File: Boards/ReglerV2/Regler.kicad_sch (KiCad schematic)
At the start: 22 parts, among them J1 In_1, J10 Ch2_LED, J11 VU_LED, J2 In_2, J3 12V_In, J4 VU_On, J5 Out_R, J6 Out_L, J7 VU_On, J8 Standby, J9 Ch1_LED, K1 DIPxx-2Axx-21x, K2 DIPxx-2Axx-21x, K3 DIPxx-2Axx-21x, K4 DIPxx-2Axx-21x, SW1 Input, SW2 VU_On, SW3 Standby

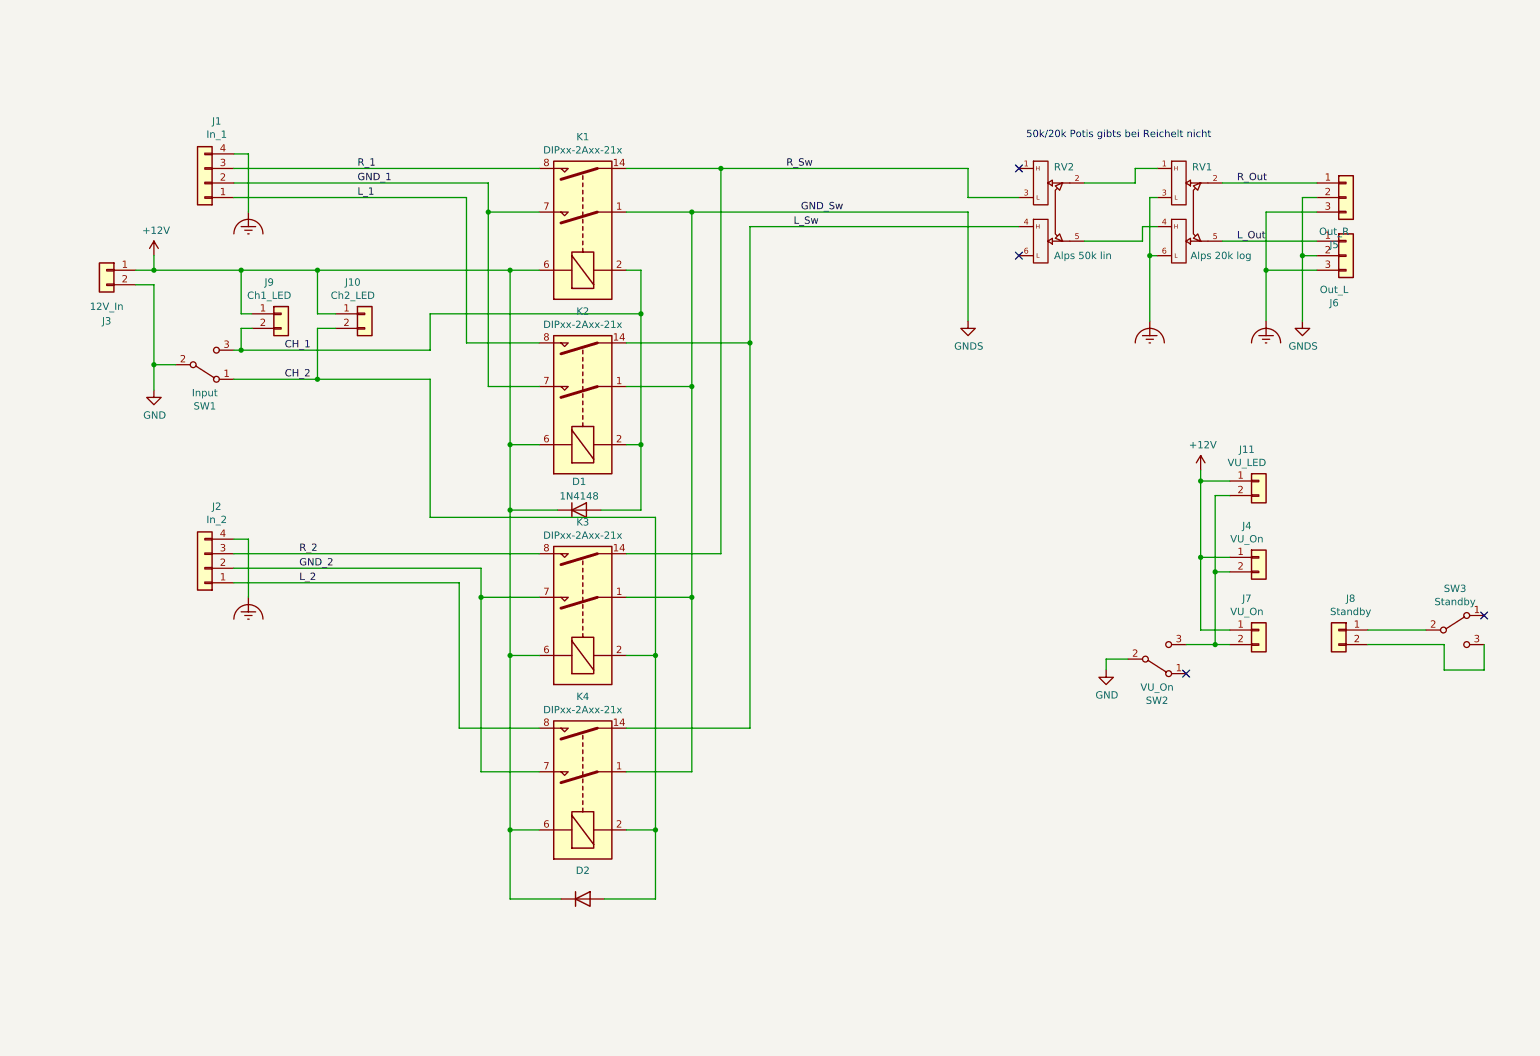
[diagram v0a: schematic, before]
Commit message: Leiterplatte erstellt
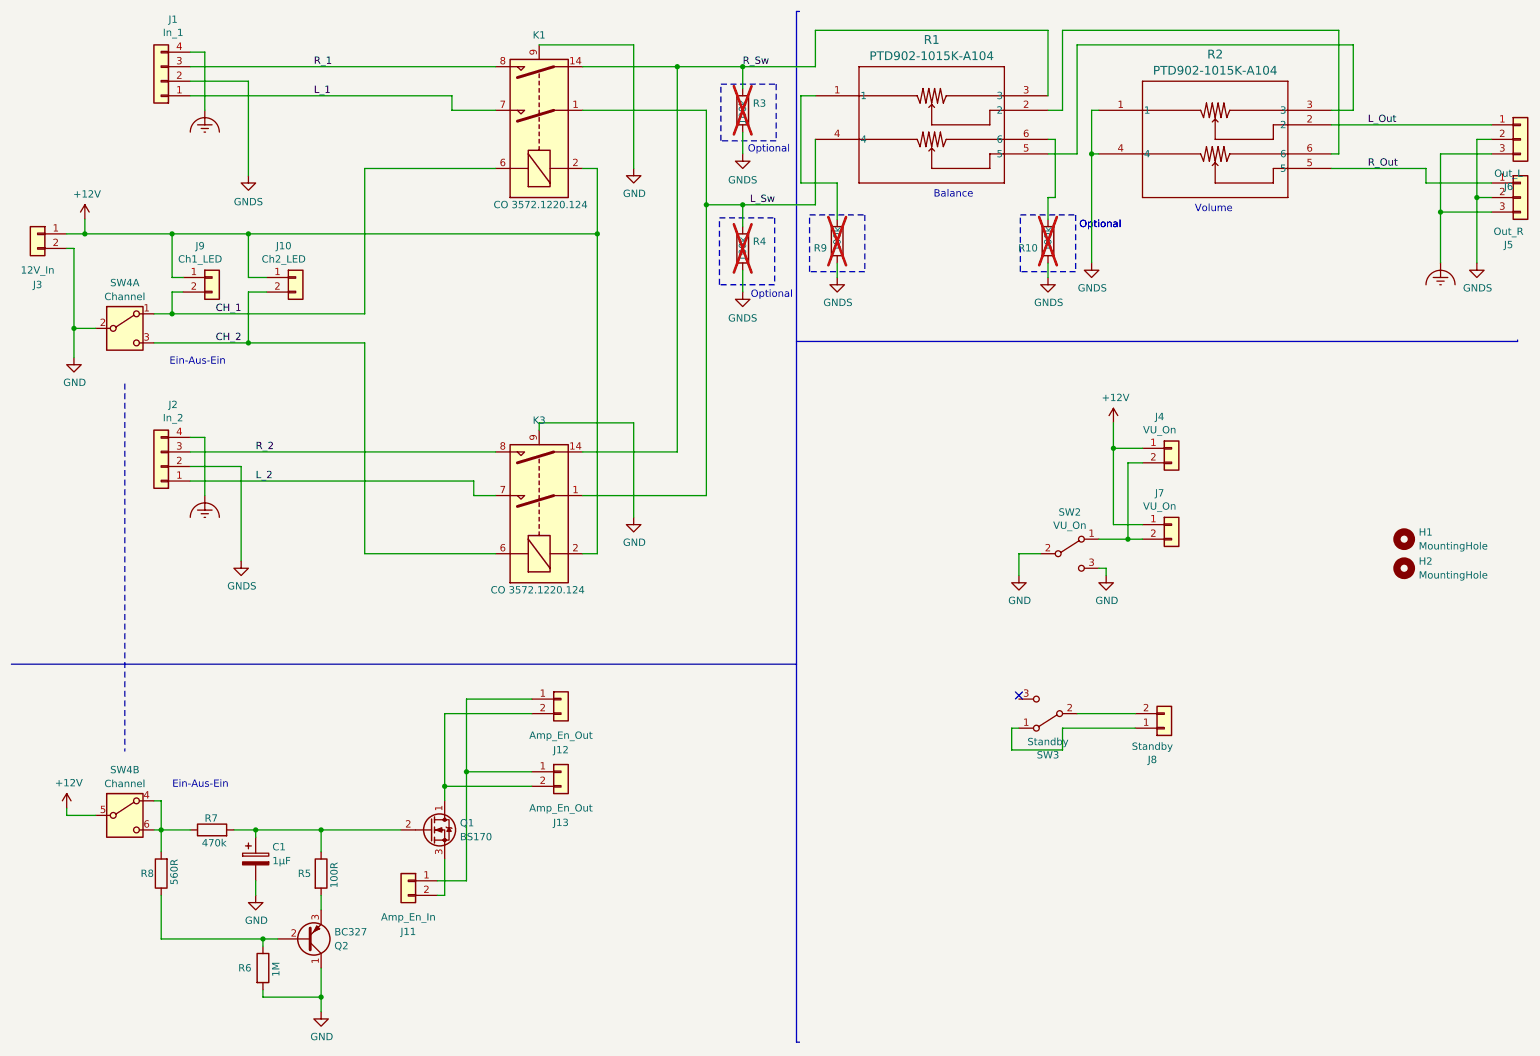
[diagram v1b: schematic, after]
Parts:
- removed D1: 1N4148, Diode_THT:D_DO-35_SOD27_P7.62mm_Horizontal, symbol Diode:1N4148
- removed D2: (no value), symbol Diode:1N4148
- removed K2, K4: DIPxx-2Axx-21x, Relay_THT:Relay_StandexMeder_DIP_LowProfile, symbol Relay:DIPxx-2Axx-21x
- removed RV1: Alps 20k log, Potentiometer_Alps_RKxxx:Potentiometer_Alps-RK271-double, symbol Regler-rescue:DUAL_POT
- removed RV2: Alps 50k lin, Potentiometer_Alps_RKxxx:Potentiometer_Alps-RK271-double, symbol Regler-rescue:DUAL_POT
- removed SW1: Input, Switch_Angled:7101MD9ABE, symbol Switch:SW_SPDT
- added C1: 1µF, Capacitor_THT:C_Rect_L4.6mm_W5.5mm_P2.50mm_MKS02_FKP02, symbol Device:C_Polarized
- added H1, H2: MountingHole, MountingHole:MountingHole_3.2mm_M3, symbol Mechanical:MountingHole
- added J12, J13: Amp_En_Out, Connector_Molex:Molex_KK-254_AE-6410-02A_1x02_P2.54mm_Vertical, symbol Connector_Generic:Conn_01x02
- added Q1: BS170, Package_TO_SOT_THT:TO-92_Inline, symbol Transistor_FET:BS170
- added Q2: BC327, Package_TO_SOT_THT:TO-92_Inline, symbol Transistor_BJT:BC327
- added R1, R2: PTD902-1015K-A104, PTD902-15K_BRN:PTD902-15K_BRN, symbol 2024-12-17_23-53-22:PTD902-1015K-A104
- added R10, R3, R4, R9: 100k, Resistor_THT:R_Axial_DIN0207_L6.3mm_D2.5mm_P10.16mm_Horizontal, symbol Device:R
- added R5: 100R, Resistor_THT:R_Axial_DIN0207_L6.3mm_D2.5mm_P10.16mm_Horizontal, symbol Device:R
- added R6: 1M, Resistor_THT:R_Axial_DIN0207_L6.3mm_D2.5mm_P10.16mm_Horizontal, symbol Device:R
- added R7: 470k, Resistor_THT:R_Axial_DIN0207_L6.3mm_D2.5mm_P10.16mm_Horizontal, symbol Device:R
- added R8: 560R, Resistor_THT:R_Axial_DIN0207_L6.3mm_D2.5mm_P10.16mm_Horizontal, symbol Device:R
- added SW4: Channel, Switch_TE:1825139-2, symbol Switch:SW_DPDT_x2
- J11: value VU_LED -> Amp_En_In
- K1, K3: value DIPxx-2Axx-21x -> CO 3572.1220.124
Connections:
- net +12V: now also K1.2, K3.2, SW4.5 (B); no longer J11.1 (Pin_1), K1.6, K3.6
- net CH_1: now also K1.6, SW4.1 (A); no longer K1.2
- net CH_2: now also K3.6, SW4.3 (C); no longer K3.2
- net GND: now also K1.9, K3.9, SW2.3 (C), C1.2, Q2.1 (C), R6.2, SW4.2 (B)
- net GNDS: now also J1.2 (Pin_2), J2.2 (Pin_2), R10.1, R2.1, R2.4, R3.2, R4.2, R9.1; no longer K1.1, K3.1
- net L_1: now also K1.7
- net L_2: now also K3.7
- net L_Out: now also R2.2
- net L_Sw: now also K1.1, K3.1, R1.4, R4.1
- net R_Out: now also R2.5
- net R_Sw: now also R1.3, R3.1
- net at J8.1 (Pin_1): now also SW3.1 (A); no longer SW3.2 (B)
- net at J8.2 (Pin_2): now also SW3.2 (B); no longer SW3.3 (C)
- net at J4.2 (Pin_2), J7.2 (Pin_2): now also SW2.1 (A); no longer J11.2 (Pin_2), SW2.3 (C)
- removed net GND_1: J1.2 (Pin_2), K1.7
- removed net GND_2: J2.2 (Pin_2), K3.7
- new net: Q2.2 (B), R6.1, R8.1
- new net: R1.5, R2.3
- new net: R1.2, R2.6
- new net: J11.1 (Pin_1), J12.1 (Pin_1), J13.1 (Pin_1)
- new net: J12.2 (Pin_2), J13.2 (Pin_2), Q1.1 (D)
- new net: R1.1, R9.2
- new net: R1.6, R10.2
- new net: C1.1, Q1.2 (G), R5.1, R7.2
- new net: Q2.3 (E), R5.2
- new net: J11.2 (Pin_2), Q1.3 (S)
- new net: R7.1, R8.2, SW4.4 (A), SW4.6 (C)
- no-connect marks 4 -> 1
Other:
- note added: "Balance"
- note added: "Ein-Aus-Ein"
- note added: "Optional"
- note added: "Volume"
- note removed: "50k/20k Potis gibts bei Reichelt nicht"
- moved on the sheet: J1, J10, J2, J3, J4, J5, J6, J7, J8, J9, SW2, SW3
